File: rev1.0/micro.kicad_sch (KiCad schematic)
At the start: 37 parts, among them J1 USB, J2 ISP, J3 Conn_01x02, J4 Conn_01x03, J5 Conn_01x04, J6 Conn_01x05, J7 Conn_01x16, Q1 FDS9926A, U1 USBLC6-2SC6, U2 ATMEGA32U4, Y1 16MHz

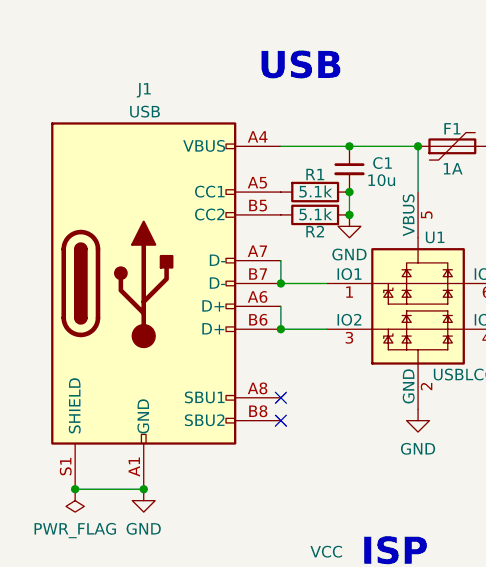
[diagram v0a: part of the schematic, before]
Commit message: updated README
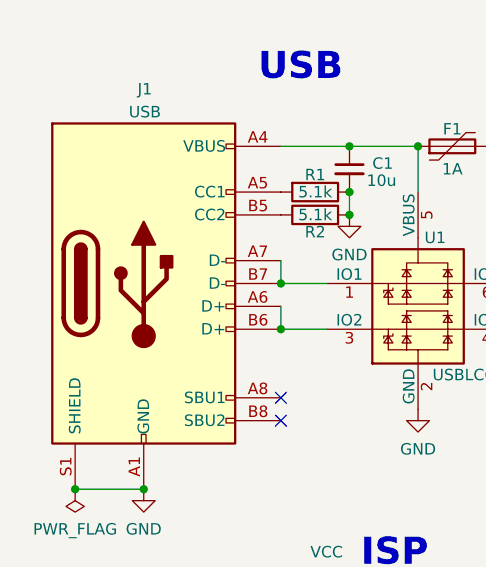
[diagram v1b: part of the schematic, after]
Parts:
- H1, H2: footprint MountingHole:MountingHole_2.2mm_M2_DIN965_Pad_TopBottom -> 0xcb:MountingHole_2.2mm_M2_DIN965_Pad_TopBottom_SMOL; now left out of the parts list
- J2: now left out of the parts list
